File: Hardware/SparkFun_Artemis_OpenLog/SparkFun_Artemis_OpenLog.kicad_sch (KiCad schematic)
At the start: 88 parts, among them J11 Qwiic_RA, J14 SWD, J2 Conn_01x02, J3 Conn_01x02, J4 Conn_01x06, J5 JST_2mm_LiPo, J6 MICRO-SD, J7 Conn_01x01, J8 USB_C_Receptacle, Q2 DMG2305UX, SW3 SMD_4.6x2.8mm_h2.5mm, U1 3.0V Supervisor, U10 CH340E, U2 MCP73831, U3 AP2112K-3.3, U4 AP2112K-3.3, U5 BNO086, U8 Artemis Module, Y1 32.768kHz, Y3 32.768kHz

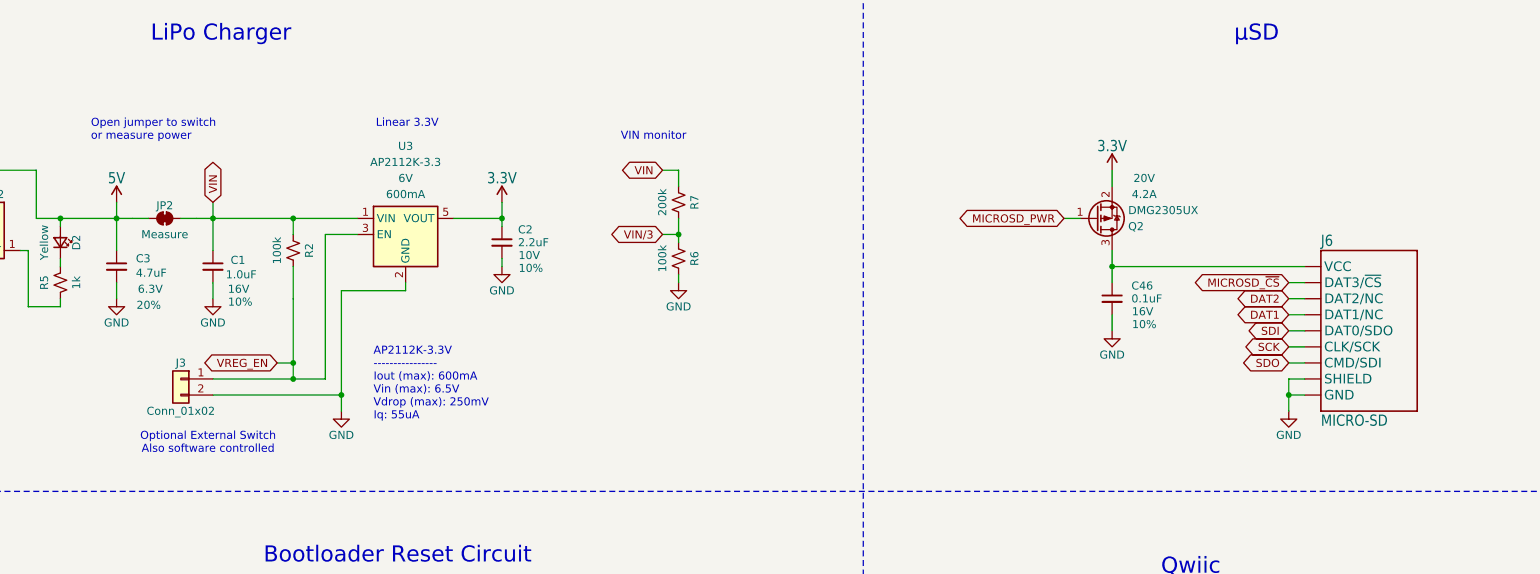
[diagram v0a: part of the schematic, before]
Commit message: Updates microSD - save point
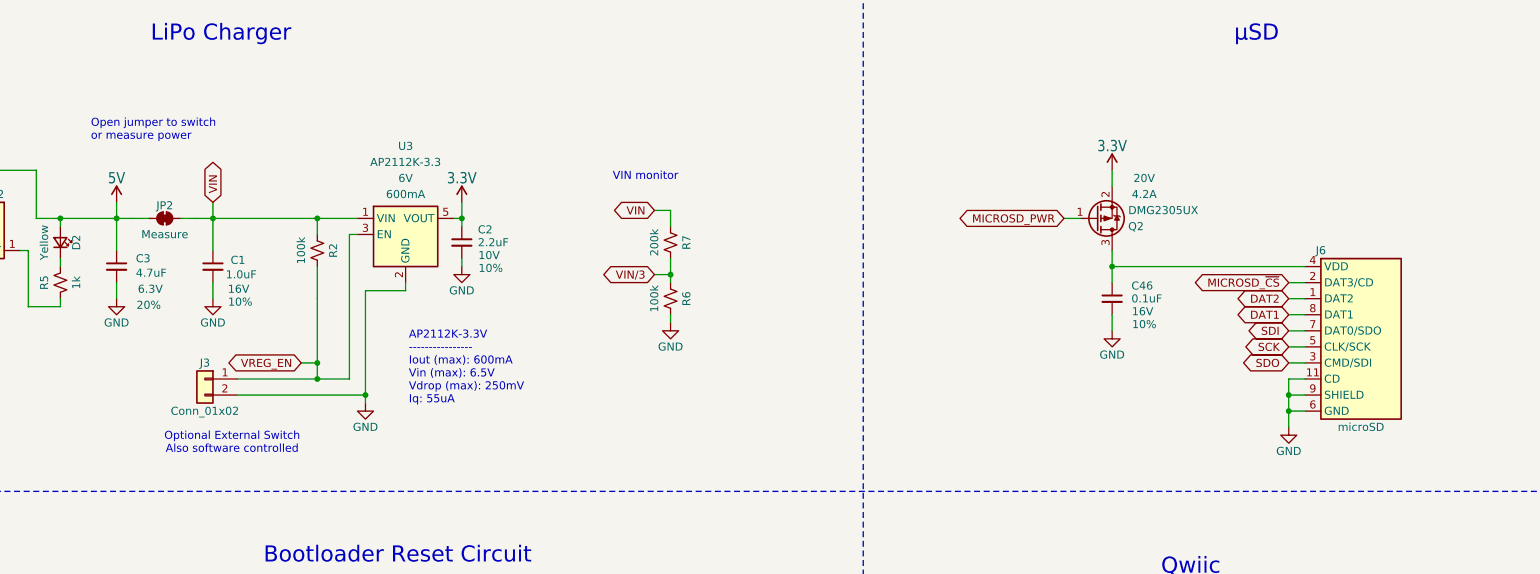
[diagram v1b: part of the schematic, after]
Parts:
- J6: value MICRO-SD -> microSD; footprint SparkFun_Artemis_OpenLog:MICRO-SD-SOCKET -> SparkFun-Connector:microSD_SOCKET; symbol SparkFun_Artemis_OpenLog-eagle-import:MICRO-SD-SDIOPUSH-PUSH -> SparkFun-Connector:microSD_PushPush_No_Drill
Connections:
- net DAT1: now also J6.8 (DAT1); no longer J6.DAT1 (DAT1/NC)
- net DAT2: now also J6.1 (DAT2); no longer J6.DAT2 (DAT2/NC)
- net GND: now also J6.10 (GND), J6.11 (CD), J6.12 (CD), J6.6 (GND), J6.9 (SHIELD); no longer J6.CD1 (SHIELD), J6.GND, J6.GND1 (GND), J6.GND3 (GND)
- net MICROSD_~{CS}: now also J6.2 (DAT3/CD); no longer J6.CS/DAT3 (DAT3/~{CS})
- net SCK: now also J6.5 (CLK/SCK); no longer J6.SCLK (CLK/SCK)
- net SDI: now also J6.7 (DAT0/SDO); no longer J6.DO/DAT0 (DAT0/SDO)
- net SDO: now also J6.3 (CMD/SDI); no longer J6.DI/CMD (CMD/SDI)
- net at C46.1, Q2.3 (D): now also J6.4 (VDD); no longer J6.VCC
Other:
- note removed: "Linear 3.3V"
- moved on the sheet: C2, J3, R2, R6, R7

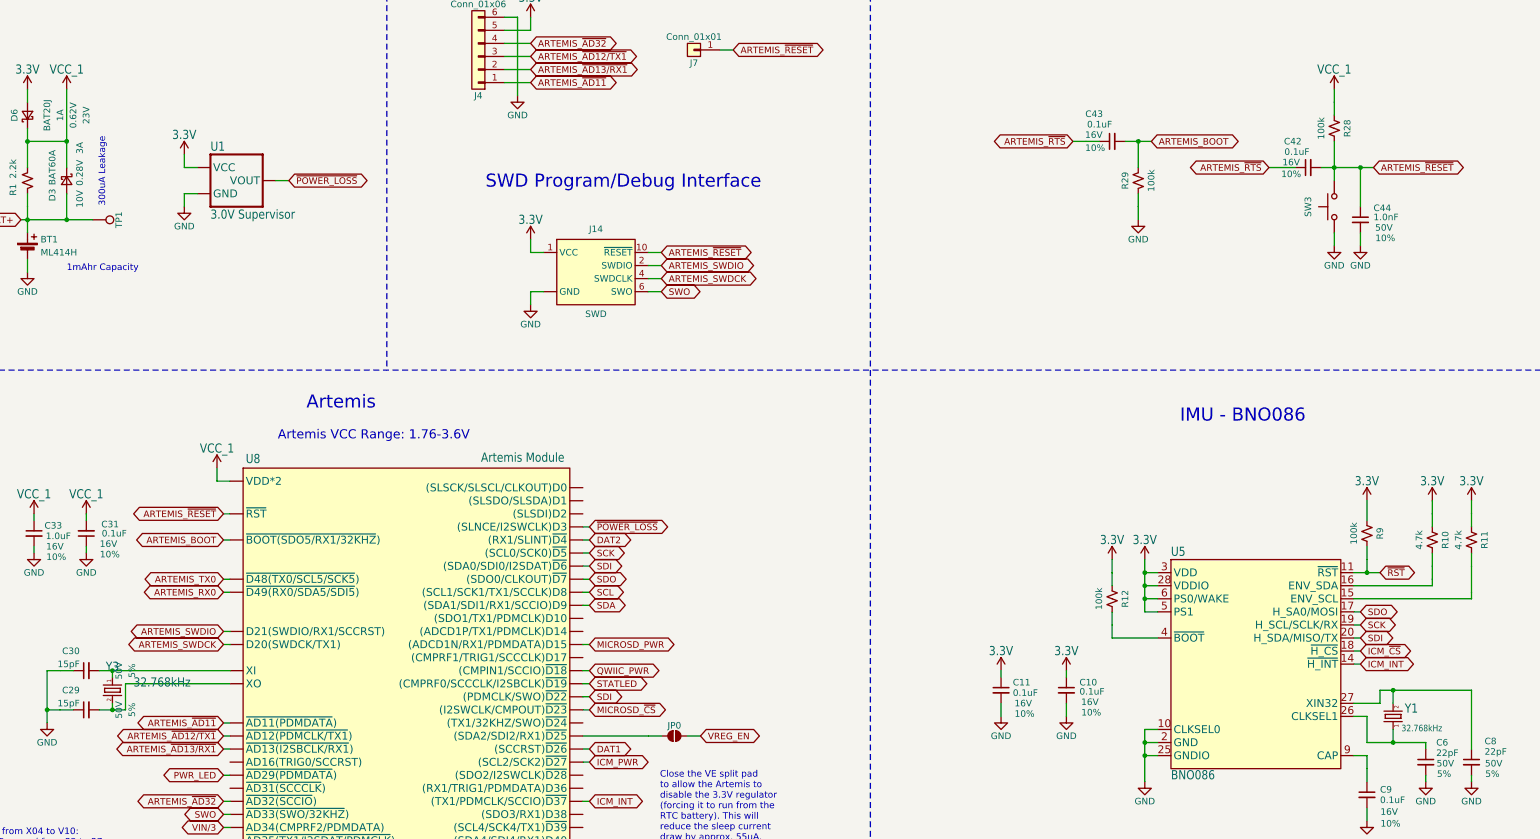
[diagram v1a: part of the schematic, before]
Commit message: All KiCad components - save point
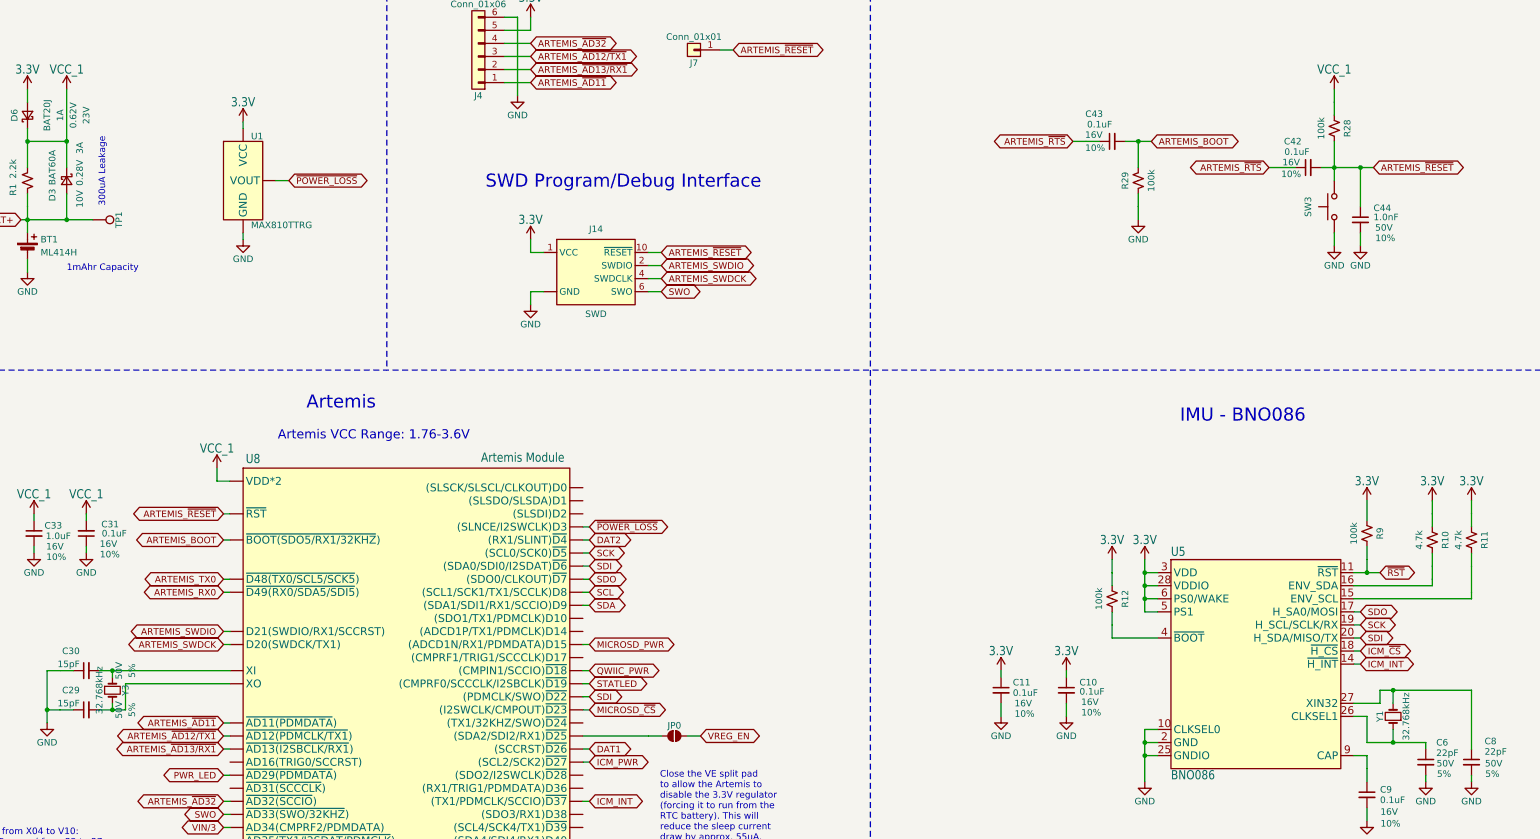
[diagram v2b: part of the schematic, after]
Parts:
- U1: value 3.0V Supervisor -> MAX810TTRG; footprint SparkFun_Artemis_OpenLog:SOT23-3 -> SparkFun-Semiconductor-Standard:SOT23-3; symbol SparkFun_Artemis_OpenLog-eagle-import:V_SUPERVISOR -> SparkFun-IC-Power:MAX810TTRG
- Y1, Y3: footprint SparkFun_Artemis_OpenLog:CRYSTAL-SMD-3.2X1.5MM -> SparkFun-Clock:Crystal_SMD_3.2x1.5mm; symbol SparkFun_Artemis_OpenLog-eagle-import:CRYSTAL-32.768KHZSMD-3.2X1.5 -> SparkFun-Clock:Crystal_32.768kHz_3.2x1.5mm; PROD_ID XTAL-13062 -> XTAL-25022
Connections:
- net at C6.1, U5.26 (CLKSEL1): now also Y1.1; no longer Y1.P$1 (1)
- net at C8.1, U5.27 (XIN32): now also Y1.2; no longer Y1.P$2 (2)
- net at C30.2, U8.XI: now also Y3.1; no longer Y3.P$1 (1)
- net at C29.2, U8.XO: now also Y3.2; no longer Y3.P$2 (2)
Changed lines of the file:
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@@
 	(wire
 		(pts
-			(xy 72.39 143.51) (xy 69.85 143.51)
-		)
-		(stroke
-			(width 0.1524)
-			(type solid)
-		)
-	)
-	(wire
-		(pts
 			(xy 76.2 287.02) (xy 78.74 287.02)
 		)
@@
 	(wire
 		(pts
-			(xy 69.85 148.59) (xy 69.85 151.13)
-		)
-		(stroke
-			(width 0.1524)
-			(type solid)
-		)
-	)
-	(wire
-		(pts
 			(xy 264.16 55.88) (xy 264.16 60.96)
 		)
@@
 	(wire
 		(pts
-			(xy 69.85 140.97) (xy 69.85 143.51)
+			(xy 81.28 134.62) (xy 81.28 135.89)
 		)
 		(stroke
@@
 	(wire
 		(pts
+			(xy 81.28 156.21) (xy 81.28 157.48)
+		)
+		(stroke
+			(width 0)
+			(type default)
+		)
+	)
+	(wire
+		(pts
 			(xy 320.04 218.44) (xy 320.04 220.98)
 		)
@@
 	(wire
 		(pts
-			(xy 72.39 148.59) (xy 69.85 148.59)
-		)
-		(stroke
-			(width 0.1524)
-			(type solid)
-		)
-	)
-	(wire
-		(pts
 			(xy 207.01 58.42) (xy 207.01 66.04)
 		)
@@
 	(symbol
 		(lib_id "SparkFun-PowerSymbol:GND")
-		(at 69.85 151.13 0)
+		(at 81.28 157.48 0)
 		(unit 1)
 		(body_style 1)
@@
 		(dnp no)
 		(property "Reference" "#PWR8"
-			(at 69.85 157.48 0)
+			(at 81.28 163.83 0)
 			(hide yes)
 			(show_name no)
@@
 		)
 		(property "Value" "GND"
-			(at 69.85 154.94 0)
+			(at 81.28 161.29 0)
 			(show_name no)
 			(do_not_autoplace yes)
@@
 		)
 		(property "Footprint" ""
-			(at 69.85 151.13 0)
+			(at 81.28 157.48 0)
 			(hide yes)
 			(show_name no)
@@
 		)
 		(property "Datasheet" ""
-			(at 69.85 151.13 0)
+			(at 81.28 157.48 0)
 			(hide yes)
 			(show_name no)
@@
 		)
 		(property "Description" "Power symbol creates a global label with name \"GND\" , ground"
-			(at 69.85 160.02 0)
+			(at 81.28 166.37 0)
 			(hide yes)
 			(show_name no)
@@
 	)
 	(symbol
-		(lib_id "SparkFun_Artemis_OpenLog-eagle-import:CRYSTAL-32.768KHZSMD-3.2X1.5")
+		(lib_id "SparkFun-Clock:Crystal_32.768kHz_3.2x1.5mm")
 		(at 304.8 250.19 90)
 		(unit 1)
@@
 		(dnp no)
 		(property "Reference" "Y1"
-			(at 308.356 249.682 90)
+			(at 302.26 250.19 0)
 			(show_name no)
 			(do_not_autoplace no)
 			(effects
 				(font
-					(size 1.778 1.5113)
+					(size 1.27 1.27)
 				)
-				(justify top)
 			)
 		)
 		(property "Value" "32.768kHz"
-			(at 310.388 253.238 90)
+			(at 307.34 250.19 0)
 			(show_name no)
 			(do_not_autoplace no)
 			(effects
 				(font
-					(size 1.27 1.0795)
+					(size 1.27 1.27)
 				)
-				(justify top)
 			)
 		)
-		(property "Footprint" "SparkFun_Artemis_OpenLog:CRYSTAL-SMD-3.2X1.5MM"
-			(at 304.8 250.19 0)
+		(property "Footprint" "SparkFun-Clock:Crystal_SMD_3.2x1.5mm"
+			(at 312.42 250.19 0)
 			(hide yes)
 			(show_name no)
@@
 			)
 		)
-		(property "Datasheet" ""
-			(at 304.8 250.19 0)
+		(property "Datasheet" "https://abracon.com/Resonators/ABS07.pdf"
+			(at 309.88 250.19 0)
 			(hide yes)
 			(show_name no)
@@
 			)
 		)
-		(property "Description" ""
-			(at 304.8 250.19 0)
+		(property "Description" "Crystal"
+			(at 317.5 250.19 0)
 			(hide yes)
 			(show_name no)
@@
 			)
 		)
-		(property "PROD_ID" "XTAL-13062"
-			(at 304.8 255.27 0)
+		(property "PROD_ID" "XTAL-25022"
+			(at 314.96 250.19 0)
 			(hide yes)
 			(show_name no)
@@
 			)
 		)
-		(pin "P$1"
+		(pin "1"
 		)
-		(pin "P$2"
+		(pin "2"
 		)
 		(instances
@@
 	)
 	(symbol
-		(lib_id "SparkFun_Artemis_OpenLog-eagle-import:V_SUPERVISOR")
-		(at 80.01 146.05 0)
+		(lib_id "SparkFun-IC-Power:MAX810TTRG")
+		(at 81.28 146.05 0)
 		(unit 1)
 		(body_style 1)
@@
 		(dnp no)
 		(property "Reference" "U1"
-			(at 74.93 140.462 0)
+			(at 82.804 138.176 0)
 			(show_name no)
 			(do_not_autoplace no)
 			(effects
 				(font
-					(size 1.778 1.5113)
+					(size 1.27 1.27)
 				)
 				(justify left bottom)
 			)
 		)
-		(property "Value" "3.0V Supervisor"
-			(at 74.93 153.67 0)
+		(property "Value" "MAX810TTRG"
+			(at 82.804 155.448 0)
 			(show_name no)
 			(do_not_autoplace no)
 			(effects
 				(font
-					(size 1.778 1.5113)
+					(size 1.27 1.27)
 				)
 				(justify left bottom)
 			)
 		)
-		(property "Footprint" "SparkFun_Artemis_OpenLog:SOT23-3"
-			(at 80.01 146.05 0)
+		(property "Footprint" "SparkFun-Semiconductor-Standard:SOT23-3"
+			(at 81.788 179.578 0)
 			(hide yes)
 			(show_name no)
@@
 			)
 		)
-		(property "Datasheet" ""
-			(at 80.01 146.05 0)
+		(property "Datasheet" "https://www.farnell.com/datasheets/89200.pdf"
+			(at 80.264 170.434 0)
 			(hide yes)
 			(show_name no)
@@
 			)
 		)
-		(property "Description" ""
-			(at 80.01 146.05 0)
+		(property "Description" "The MAX809 and MAX810 are cost−effective system supervisor circuits designed to monitor VCC in digital systems and provide a reset signal to the host processor when necessary. No external components are required."
+			(at 82.042 167.64 0)
 			(hide yes)
 			(show_name no)
@@
 		)
 		(property "PROD_ID" "IC-14809"
-			(at 80.01 156.718 0)
+			(at 81.28 177.8 0)
 			(hide yes)
 			(show_name no)
@@
 	(symbol
 		(lib_id "SparkFun_Artemis_OpenLog-eagle-import:3.3V")
-		(at 69.85 140.97 0)
+		(at 81.28 134.62 0)
 		(unit 1)
 		(body_style 1)
@@
 		(dnp no)
 		(property "Reference" "#SUPPLY4"
-			(at 69.85 140.97 0)
+			(at 81.28 134.62 0)
 			(hide yes)
 			(show_name no)
@@
 		)
 		(property "Value" "3.3V"
-			(at 69.85 138.176 0)
+			(at 81.28 131.826 0)
 			(show_name no)
 			(do_not_autoplace no)
@@
 		)
 		(property "Footprint" ""
-			(at 69.85 140.97 0)
+			(at 81.28 134.62 0)
 			(hide yes)
 			(show_name no)
@@
 		)
 		(property "Datasheet" ""
-			(at 69.85 140.97 0)
+			(at 81.28 134.62 0)
 			(hide yes)
 			(show_name no)
@@
 		)
 		(property "Description" ""
-			(at 69.85 140.97 0)
+			(at 81.28 134.62 0)
 			(hide yes)
 			(show_name no)
@@
 	)
 	(symbol
-		(lib_id "SparkFun_Artemis_OpenLog-eagle-import:CRYSTAL-32.768KHZSMD-3.2X1.5")
+		(lib_id "SparkFun-Clock:Crystal_32.768kHz_3.2x1.5mm")
 		(at 55.88 245.11 270)
 		(unit 1)
@@
 		(dnp no)
 		(property "Reference" "Y3"
-			(at 55.88 241.554 90)
+			(at 58.42 245.11 0)
 			(show_name no)
 			(do_not_autoplace no)
 			(effects
 				(font
-					(size 1.778 1.5113)
+					(size 1.27 1.27)
 				)
-				(justify bottom)
 			)
 		)
 		(property "Value" "32.768kHz"
-			(at 65.532 244.602 90)
+			(at 53.34 245.11 0)
 			(show_name no)
 			(do_not_autoplace no)
 			(effects
 				(font
-					(size 1.778 1.5113)
+					(size 1.27 1.27)
 				)
-				(justify bottom)
 			)
 		)
-		(property "Footprint" "SparkFun_Artemis_OpenLog:CRYSTAL-SMD-3.2X1.5MM"
-			(at 55.88 245.11 0)
+		(property "Footprint" "SparkFun-Clock:Crystal_SMD_3.2x1.5mm"
+			(at 48.26 245.11 0)
 			(hide yes)
 			(show_name no)
@@
 			)
 		)
-		(property "Datasheet" ""
-			(at 55.88 245.11 0)
+		(property "Datasheet" "https://abracon.com/Resonators/ABS07.pdf"
+			(at 50.8 245.11 0)
 			(hide yes)
 			(show_name no)
@@
 			)
 		)
-		(property "Description" ""
-			(at 55.88 245.11 0)
+		(property "Description" "Crystal"
+			(at 43.18 245.11 0)
 			(hide yes)
 			(show_name no)
@@
 			)
 		)
-		(property "PROD_ID" "XTAL-13062"
-			(at 55.88 250.19 0)
+		(property "PROD_ID" "XTAL-25022"
+			(at 45.72 245.11 0)
 			(hide yes)
 			(show_name no)
@@
 			)
 		)
-		(pin "P$1"
+		(pin "2"
 		)
-		(pin "P$2"
+		(pin "1"
 		)
 		(instances
